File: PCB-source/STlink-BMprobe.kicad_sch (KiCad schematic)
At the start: 38 parts, among them Q700 MMST3904, U700 STM32F103CBTx, Y700 Crystal_GND24

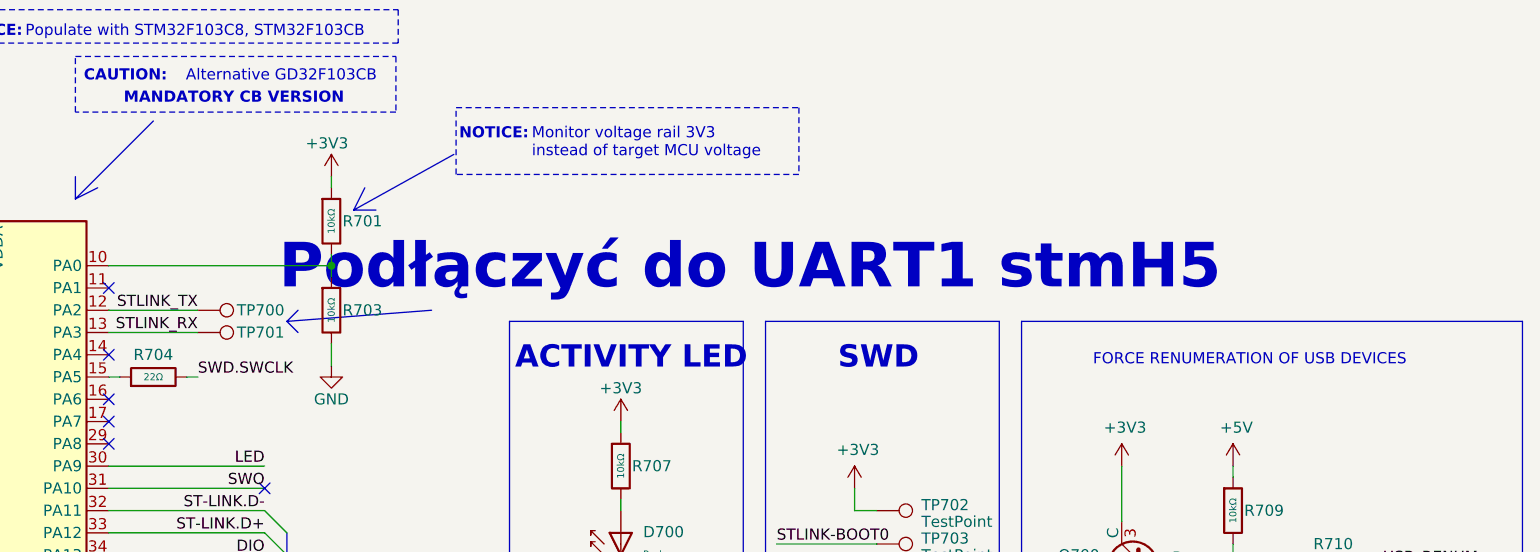
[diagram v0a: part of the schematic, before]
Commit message: in progress
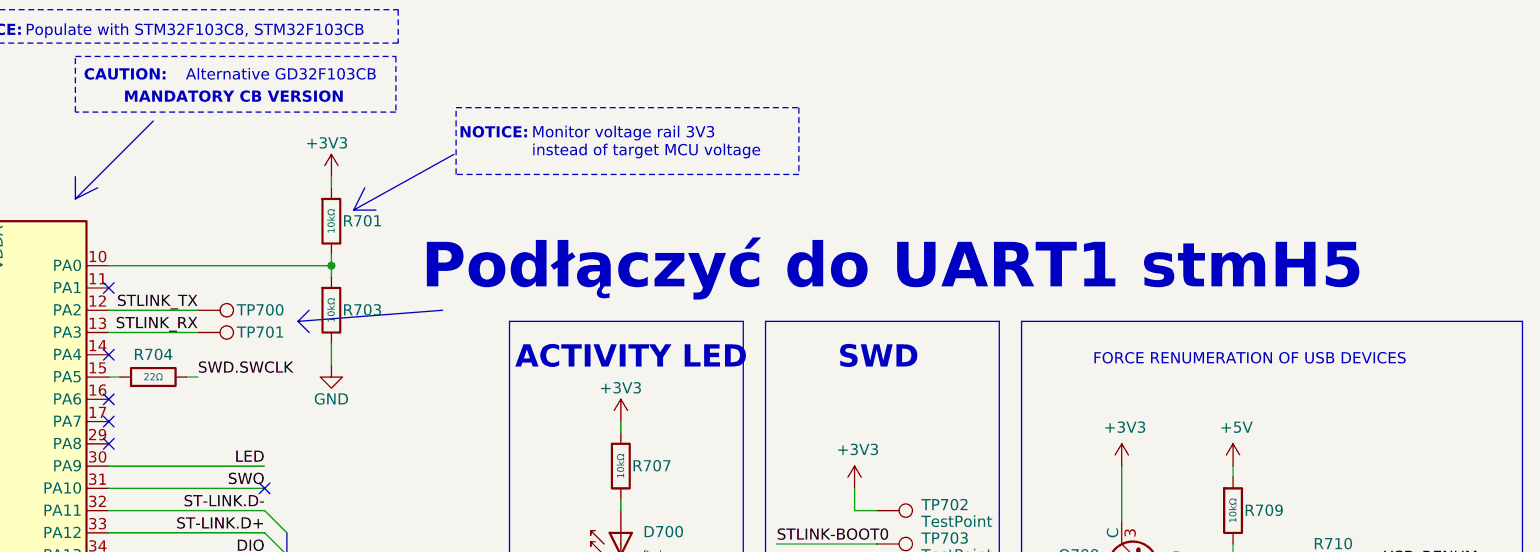
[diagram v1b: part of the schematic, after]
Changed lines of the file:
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@@
 	(text "Podłączyć do UART1 stmH5\n"
 		(exclude_from_sim no)
-		(at 189.992 62.484 0)
+		(at 206.248 62.484 0)
 		(effects
 			(font
@@
 	(polyline
 		(pts
-			(xy 153.67 67.31) (xy 137.16 68.58)
+			(xy 154.94 67.31) (xy 138.43 68.58)
 		)
 		(stroke
@@
 	(polyline
 		(pts
-			(xy 137.16 68.58) (xy 138.43 69.85)
+			(xy 138.43 68.58) (xy 139.7 69.85)
 		)
 		(stroke
@@
 	(polyline
 		(pts
-			(xy 137.16 68.58) (xy 138.43 67.31)
-		)
-		(stroke
+			(xy 138.43 68.58) (xy 139.7 67.31)
+		)
+		(stroke
